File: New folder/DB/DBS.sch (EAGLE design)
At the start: 132 parts, among them J1 TYPE-C-31-M-12, J10 TYPE-C-31-M-12, J11 TYPE-C-31-M-12, J12 TYPE-C-31-M-12, J13 TYPE-C-31-M-12, J14 TYPE-C-31-M-12, J15 TYPE-C-31-M-12, J16 TYPE-C-31-M-12, J17 TYPE-C-31-M-12, J18 TYPE-C-31-M-12, J19 TYPE-C-31-M-12, J2 TYPE-C-31-M-12, J20 TYPE-C-31-M-12, J21 TYPE-C-31-M-12, J26 TYPE-C-31-M-12, J3 TYPE-C-31-M-12, J4 TYPE-C-31-M-12, J5 TYPE-C-31-M-12, J6 TYPE-C-31-M-12, J7 TYPE-C-31-M-12, J8 TYPE-C-31-M-12, J9 TYPE-C-31-M-12, X1 SM04B-SRSS-TB, X10 SM04B-SRSS-TB, X11 SM04B-SRSS-TB, X12 SM04B-SRSS-TB, X13 SM04B-SRSS-TB, X14 SM04B-SRSS-TB, X15 SM04B-SRSS-TB, X16 SM04B-SRSS-TB, X17 SM04B-SRSS-TB, X18 SM04B-SRSS-TB, X19 SM04B-SRSS-TB, X2 SM04B-SRSS-TB, X20 SM04B-SRSS-TB, X21 SM04B-SRSS-TB, X26 SM04B-SRSS-TB, X3 SM04B-SRSS-TB, X4 SM04B-SRSS-TB, X5 SM04B-SRSS-TB, X6 SM04B-SRSS-TB, X7 SM04B-SRSS-TB, X8 SM04B-SRSS-TB, X9 SM04B-SRSS-TB

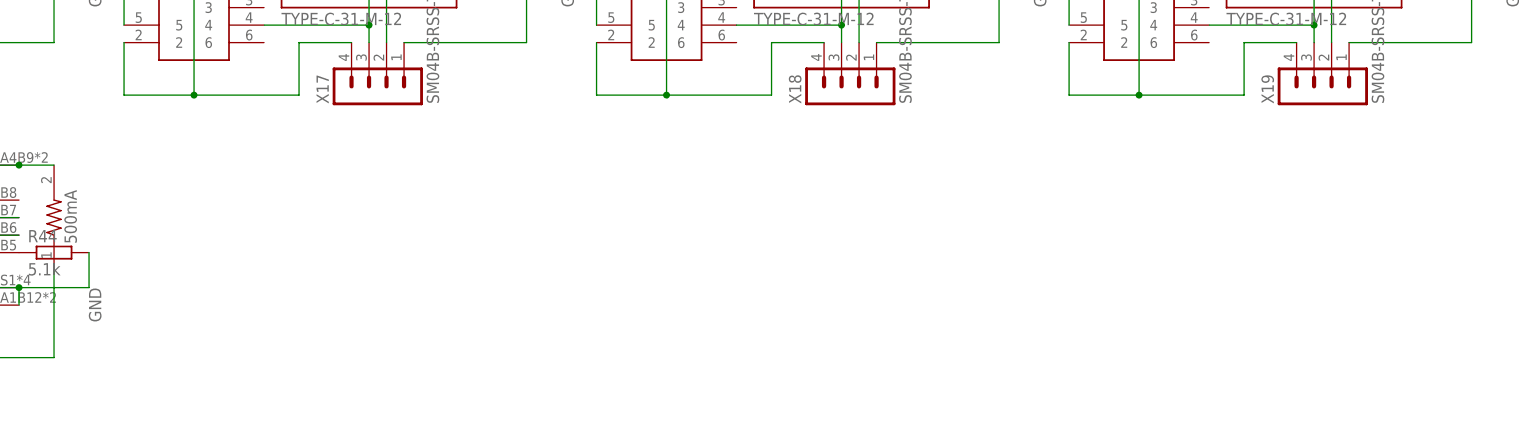
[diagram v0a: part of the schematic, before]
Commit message: add
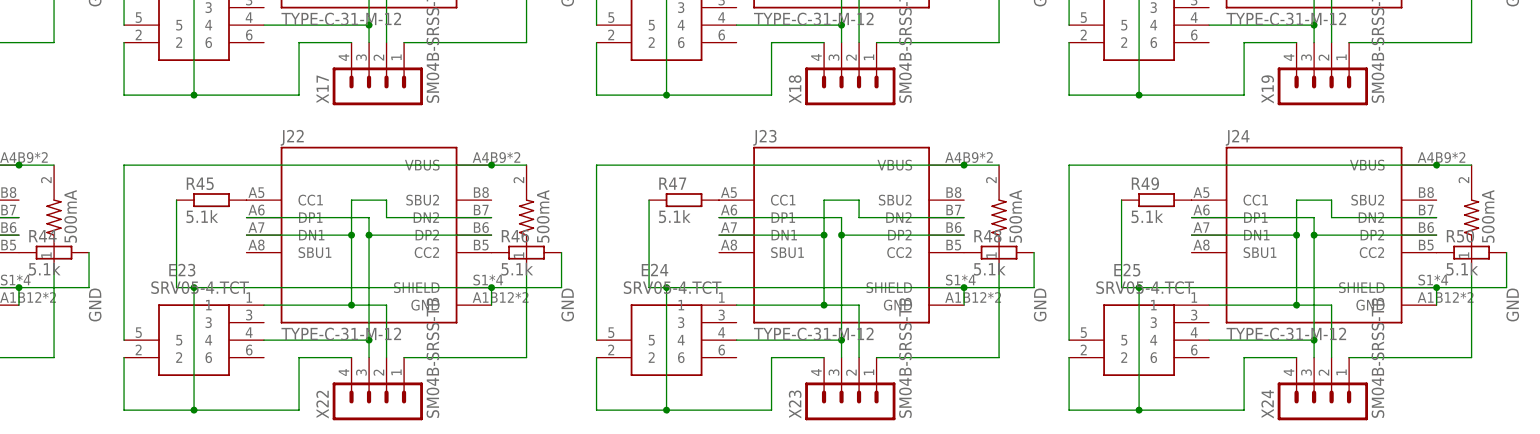
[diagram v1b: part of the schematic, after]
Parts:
- added E23, E24, E25: SRV05-4.TCT, SRV05-4.TCT:SRV05-4.TCT
- added F23, F24, F25: 500mA, fuse:0ZCJ0075AF2E
- added J22, J23, J24: TYPE-C-31-M-12, TYPE-C-31-M-12:TYPE-C-31-M-12
- added R45, R46, R47, R48, R49, R50: 5.1k, Components:RESISTOR-0603
- added X22, X23, X24: SM04B-SRSS-TB, con-JST SH:SM04B-SRSS-TB
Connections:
- new net DN23: E23.1, J22.DN1, J22.DN2, X22.2
- new net DN24: E24.1, J23.DN1, J23.DN2, X23.2
- new net DN25: E25.1, J24.DN1, J24.DN2, X24.2
- new net DP23: E23.4, J22.DP1, J22.DP2, X22.3
- new net DP24: E24.4, J23.DP1, J23.DP2, X23.3
- new net DP25: E25.4, J24.DP1, J24.DP2, X24.3
- new net N$185: E23.5, F23.2, J22.VBUS
- new net N$186: F23.1, X22.1
- new net N$187: J22.CC1, R45.2
- new net N$188: J22.CC2, R46.1
- new net N$189: E24.5, F24.2, J23.VBUS
- new net N$190: F24.1, X23.1
- new net N$191: J23.CC1, R47.2
- new net N$192: J23.CC2, R48.1
- new net N$193: E25.5, F25.2, J24.VBUS
- new net N$194: F25.1, X24.1
- new net N$195: J24.CC1, R49.2
- new net N$196: J24.CC2, R50.1
- net GND: now also E23.2, E24.2, E25.2, J22.GND, J22.SHIELD, J23.GND, J23.SHIELD, J24.GND, J24.SHIELD, R45.1, R46.2, R47.1, R48.2, R49.1, R50.2, X22.4, X23.4, X24.4
